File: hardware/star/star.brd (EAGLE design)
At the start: 116.5 x 163.8 mm, 166 parts, among them IC1 MAX481CSA, IC2 LD117AS12TR, IC22 LD117AS12TR, IC3 74HCT08D, IC4 7404D, IC5 LM317MABDT, IC6 LM317MABDT, IC7 LM317MABDT, IC8 MAX481CSA, IC9 LD117AS12TR, K1 T90-12VDC-TL-A, K2 T90-12VDC-TL-A, P1 B3B-PH-K, Q1 35A/25V/8.5mΩ, Q2 35A/25V/8.5mΩ, Q3 35A/25V/8.5mΩ, Q4 35A/25V/8.5mΩ, T1 T_PNP_MMBT5401_CHANGJ_SOT23-B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, T2 T_PNP_MMBT5401_CHANGJ_SOT23-B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, T3 T_PNP_MMBT5401_CHANGJ_SOT23-B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, T4 T_PNP_MMBT5401_CHANGJ_SOT23-B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, U1 TCLT1600, X1 MKDSN1,5/2-5,08, X3 MKDSN1,5/5-5,08

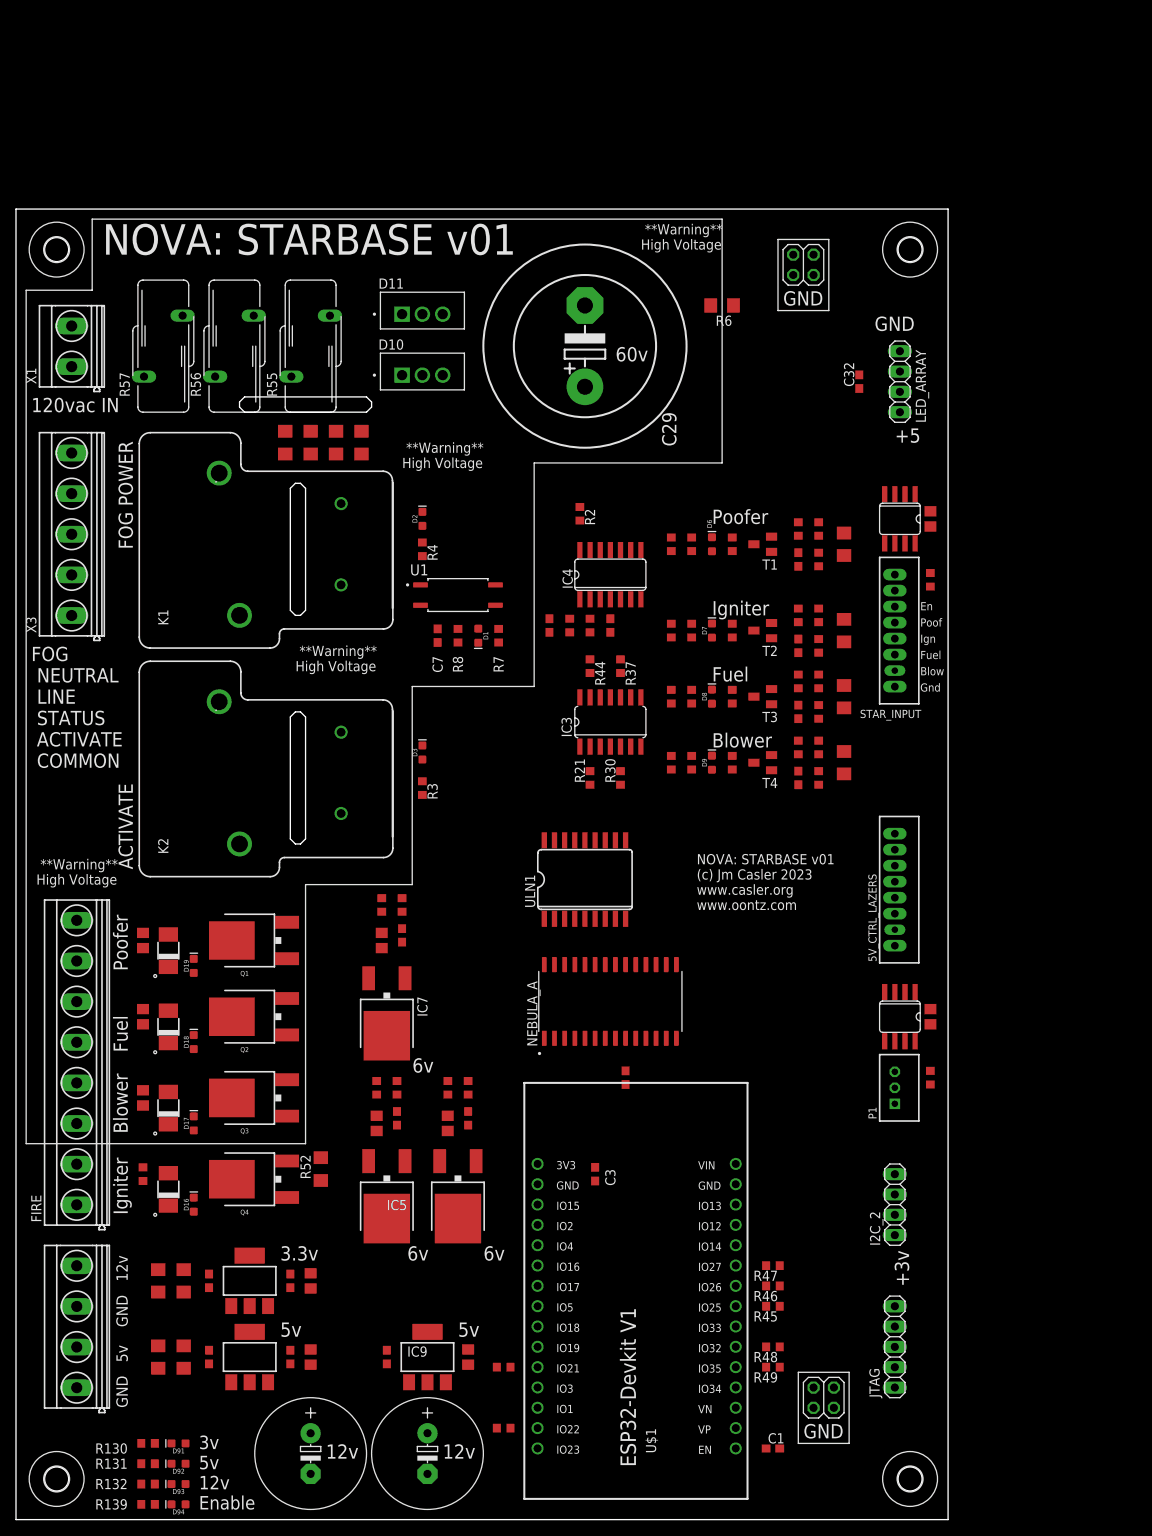
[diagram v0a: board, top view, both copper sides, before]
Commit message: Added buckboost
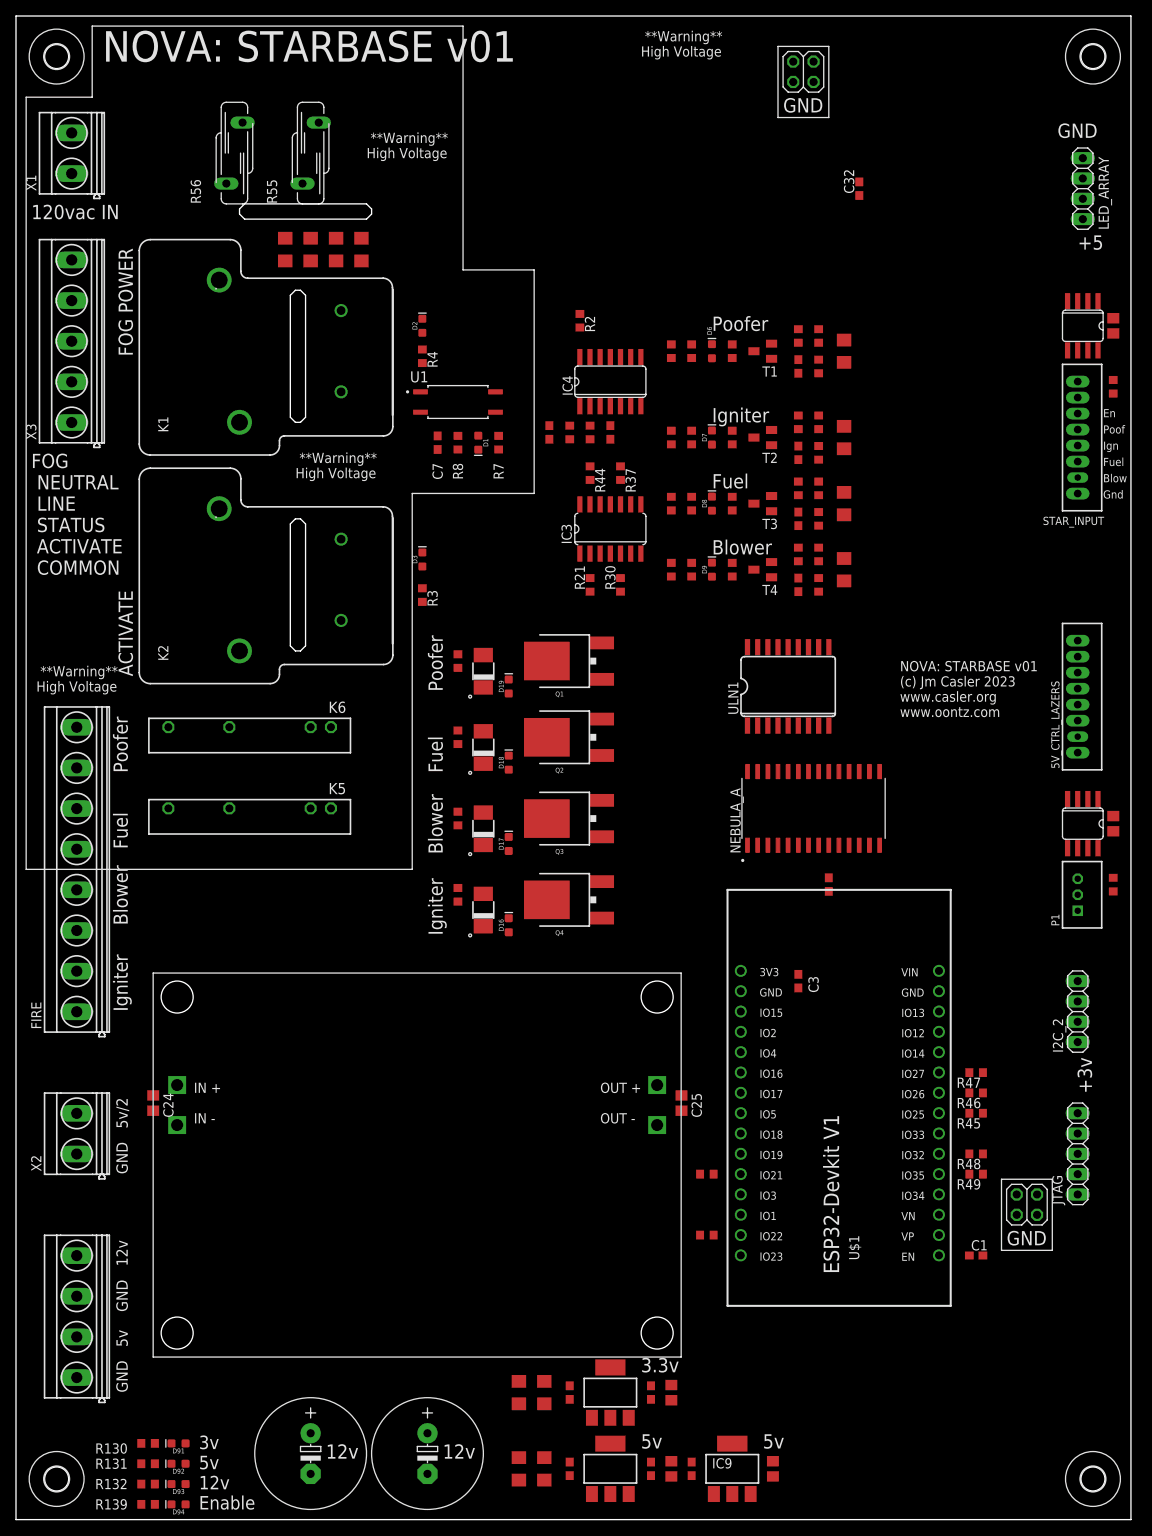
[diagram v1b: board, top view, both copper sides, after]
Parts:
- removed C26, C30: 1uf, rcl:C0805
- removed C27, C31: 10uf, rcl:C0603
- removed C29: (no value), rcl:EB25D
- removed D10, D11: MBR20200CT, MBR20200CT:TO254P1050X476X2020-3
- removed IC5, IC6, IC7: LM317MABDT, v-reg:DPACK
- removed R50, R53, R58: R_240R_0603, JLC PCB Basic Parts_loc:R0603
- removed R51, R54, R59: R_750R_0603, JLC PCB Basic Parts_loc:R0603
- removed R52, R6: R_0R_1206, JLC PCB Basic Parts_loc:R1206
- removed R57: S14K420, varistor:S14K420
- added K5, K6: AQG22110, relay:AQG
- added U$2: ZK-SJVA-4X, Nova:ZK-SJVA-4X
- added X2: MKDSN1,5/2-5,08, con-phoenix-508-jm:MKDSN1,5/2-5,08
- C25: value 10uf -> 1uf; device rcl:C0603 -> rcl:C0805
- R55, R56: value S14K420 -> S10K40; device varistor:S14K420 -> varistor:S10K40
- R60, R61: value R_56K_0805 -> R_1K_0603; device JLC PCB Basic Parts_loc:R0805 -> JLC PCB Basic Parts_loc:R0603
- R62: value R_56K_0805 -> R_7.5K_0603; device JLC PCB Basic Parts_loc:R0805 -> JLC PCB Basic Parts_loc:R0603
- R63: value R_2.2K_0603 -> R_1K_0603
- moved D12 52.6 mm to (58.4, 106.0)
- moved D13 52.6 mm to (58.4, 96.5)
- moved D14 52.6 mm to (58.4, 86.4)
- moved D15 52.6 mm to (58.4, 76.2)
- moved D16 52.6 mm to (61.6, 74.3)
- moved R61 52.6 mm to (55.2, 97.8)
- moved R63 52.6 mm to (55.2, 78.1)
- moved D17 52.6 mm to (61.6, 84.5)
- moved D18 52.6 mm to (61.6, 94.6)
- moved D19 52.6 mm to (61.6, 104.1)
- moved Q1 52.6 mm to (67.9, 107.3)
- moved Q2 52.6 mm to (67.9, 97.8)
- moved Q3 52.6 mm to (67.9, 87.6)
- moved Q4 52.6 mm to (67.9, 77.5)
- moved R60 52.6 mm to (55.2, 107.3)
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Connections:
- removed net +6V: D15.C, D16.A, FIRE.1, IC5.4, IC6.4, IC7.4, R50.2, R53.2, R58.2
- removed net 60VDC: C29.+, D10.2, D12.C, D13.C, D14.C, D17.A, D18.A, D19.A, FIRE.3, FIRE.5, FIRE.7
- removed net N$53: IC7.1, R58.1, R59.2
- new net +14V: C25.1, D14.C, D17.A, FIRE.3, U$2.OUT+
- new net +5V/2: D15.C, D16.A, FIRE.1, X2.2
- net +12V: now also U$2.IN+; no longer C25.1, C26.1, C27.1, C30.1, C31.1, IC5.3, IC6.3, IC7.3
- net +5V: now also D12.C, D13.C, D18.A, D19.A, K5.+, K6.+
- net 120_LINE: now also K5.O1, K6.O1; no longer D10.1, D10.3, R57.1
- net 120_NEUTRAL: now also FIRE.6, FIRE.8; no longer D11.2, R57.2
- net GND: now also C24.2, C25.2, Q3.3, U$2.IN-, U$2.OUT-, X2.1; no longer R52.1, R6.1
- net GND2: no longer C29.-, D11.1, D11.3, Q3.3, R6.2
- net GND3: no longer C24.2, C25.2, C26.2, C27.2, C30.2, C31.2, R51.1, R52.2, R54.1, R59.1
- net N$47: now also K5.-; no longer FIRE.6
- net N$48: now also FIRE.7, K6.O2; no longer IC6.1, R53.1, R54.2
- net N$49: now also K6.-; no longer FIRE.8
- net N$50: now also FIRE.5, K5.O2; no longer IC5.1, R50.1, R51.2
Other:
- board size 116.5 x 163.8 mm -> 139.4 x 187.9 mm
- board text added: "GND 5v/2"
- board text removed: "60v"
- board text removed: "6v"
